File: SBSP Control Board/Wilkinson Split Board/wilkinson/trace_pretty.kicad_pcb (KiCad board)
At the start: 4 copper layers, 46.4 x 134.2 mm, 77 parts, among them IC1 SN74AVC2T245RSWR, J1 Conn_01x02_Socket, J10 Conn_Coaxial, J11 Conn_Coaxial, J12 Conn_Coaxial, J13 Conn_Coaxial, J14 Conn_Coaxial, J15 Conn_Coaxial, J16 Conn_Coaxial, J17 Conn_Coaxial, J2 Conn_01x02_Socket, J3 Conn_01x20_Socket, J4 Conn_01x20_Socket, J5 Conn_01x12_Socket, J6 Conn_01x02_Pin, J7 Conn_01x02_Pin, J8 Conn_01x02_Pin, J9 Conn_Coaxial, U1 ADAR1000ACCZN, U2 SN74AVC4T245PW, U3 SN74AVC4T245PW, U4 ADAR1000ACCZN

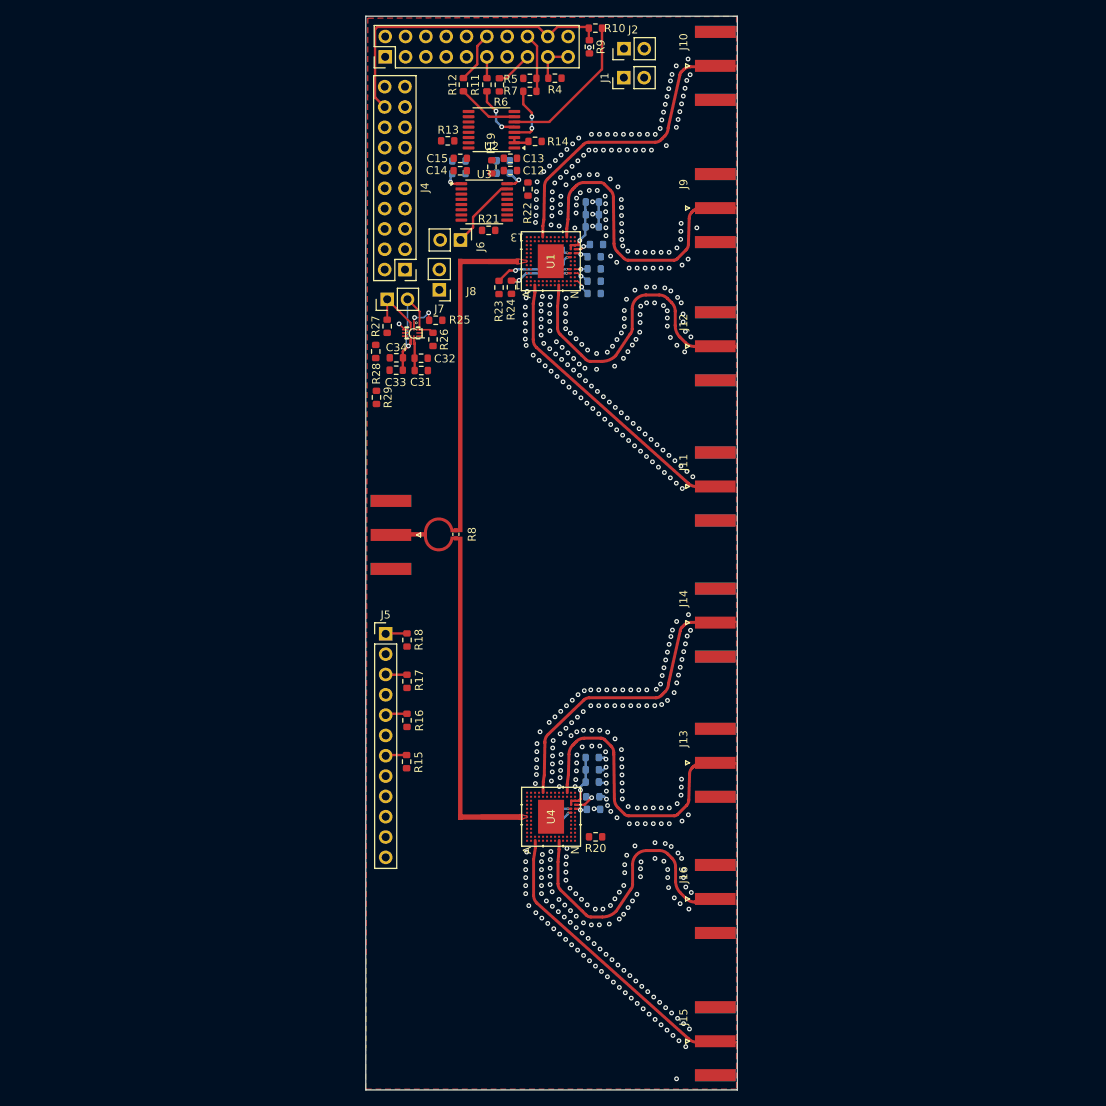
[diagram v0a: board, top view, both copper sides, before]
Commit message: gave to fayed for sims
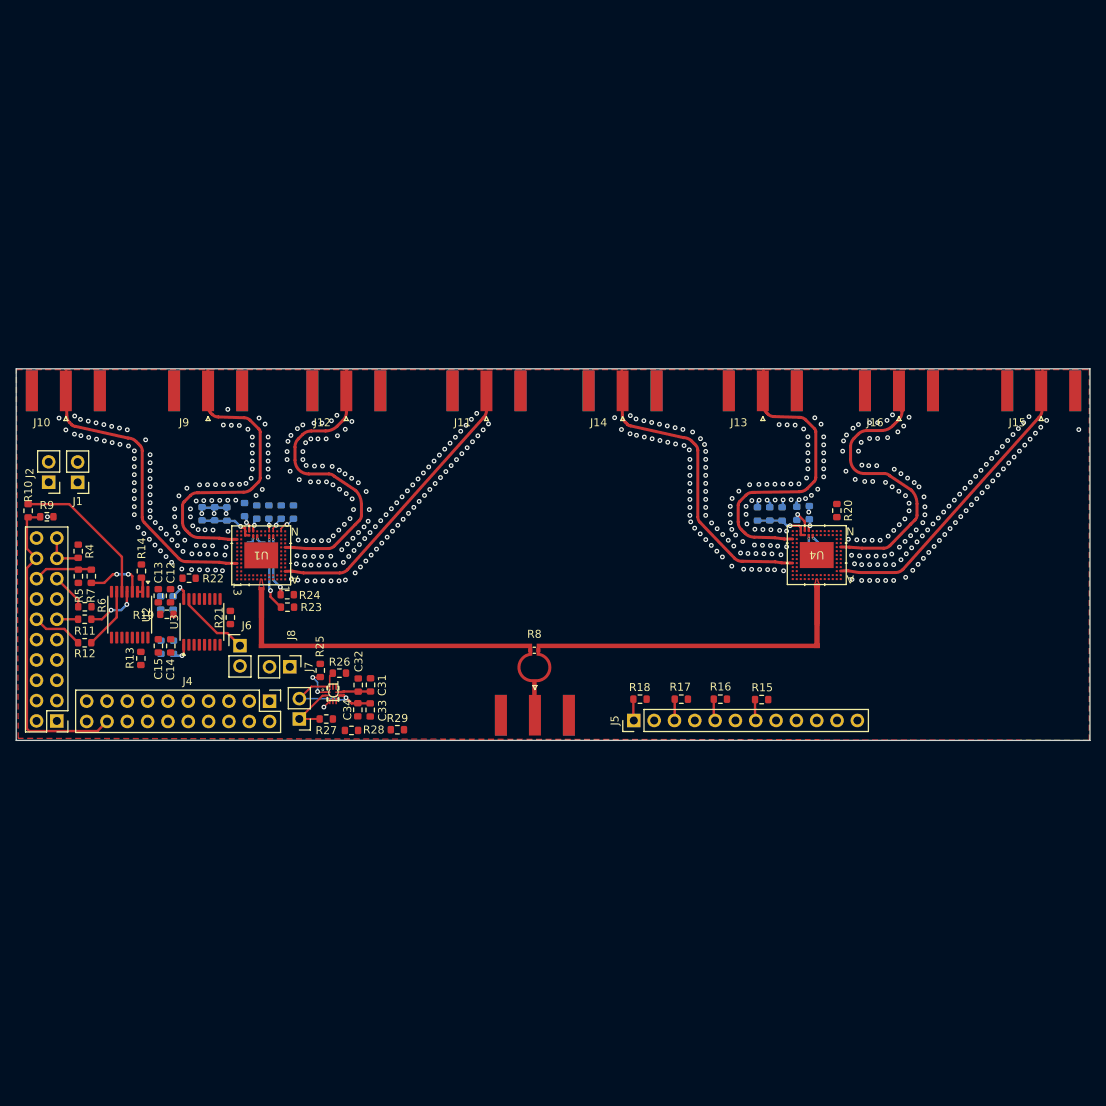
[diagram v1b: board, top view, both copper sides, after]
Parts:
- moved R10 93.1 mm to (374.2, 122.7), turned to 90 degrees
- moved J3 92.6 mm to (377.8, 148.9), turned to 180 degrees
- moved J15 90.9 mm to (500.9, 107.7), turned to 90 degrees
- moved J10 90.8 mm to (379.0, 107.7), turned to 90 degrees
- moved J2 90.0 mm to (376.8, 119.1), turned to 180 degrees
- moved R9 89.7 mm to (376.6, 123.4), turned to 0 degrees
- moved J1 85.0 mm to (380.4, 119.1), turned to 180 degrees
- moved R12 84.3 mm to (381.3, 139.2), turned to 0 degrees
- moved R5 84.0 mm to (380.5, 130.9), turned to 90 degrees
- moved R4 83.9 mm to (380.5, 127.7), turned to -90 degrees
- moved R11 83.6 mm to (381.3, 136.2), turned to 0 degrees
- moved R6 83.3 mm to (381.3, 134.7), turned to 0 degrees
- moved R7 81.7 mm to (382.1, 130.9), turned to -90 degrees
- moved U2 75.6 mm to (386.9, 135.7), turned to -90 degrees
- moved R13 75.2 mm to (388.3, 141.1), turned to -90 degrees
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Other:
- board size 46.4 x 134.2 mm -> 134.2 x 46.4 mm
